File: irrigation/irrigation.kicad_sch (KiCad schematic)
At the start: 37 parts, among them J1 24V Jmp, J10 24V, J11 25%, J12 50%, J13 75%, J14 100%, J15 100%, J16 100%, J17 Pump, J2 Power, J3 Power, J4 Power, J5 Power, J6 Power, J7 Power, J8 0V Jmp, J9 Empty, K1 PLC-RPT-24DC/21, K2 PLC-RPT-24DC/21, M1 Pump, SW1 Well Empty, SW2 100% Full, SW3 25% Full, SW4 50% Full, SW5 75% Full, U1 MPPT-Charger

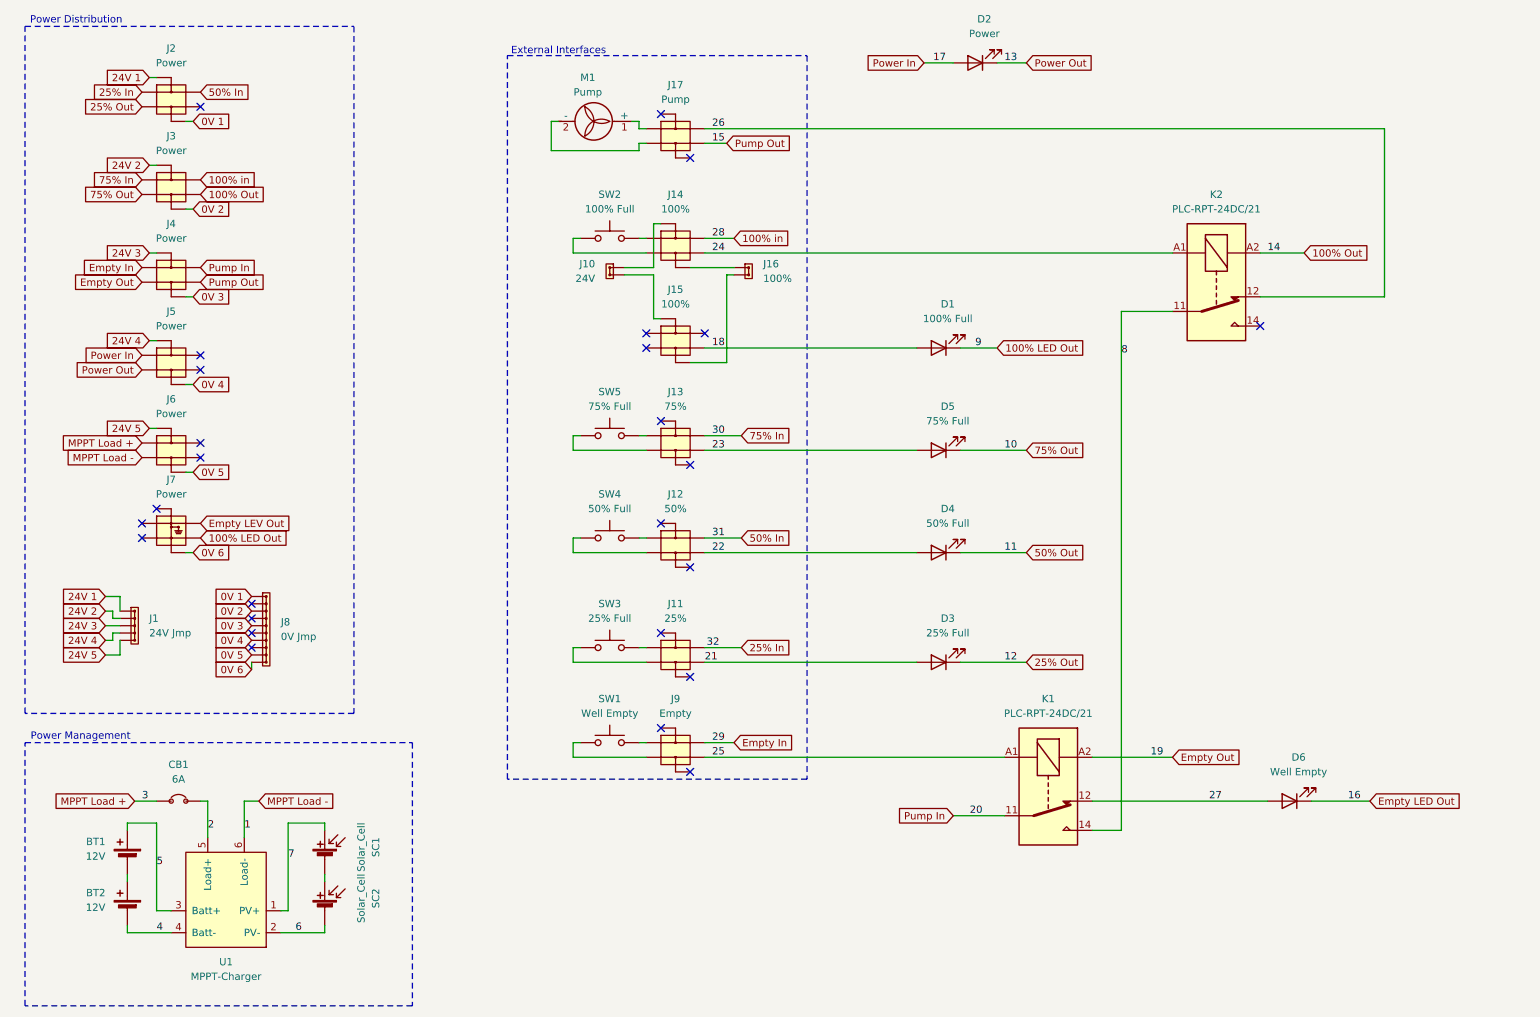
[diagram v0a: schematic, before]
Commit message: Attempting to organize
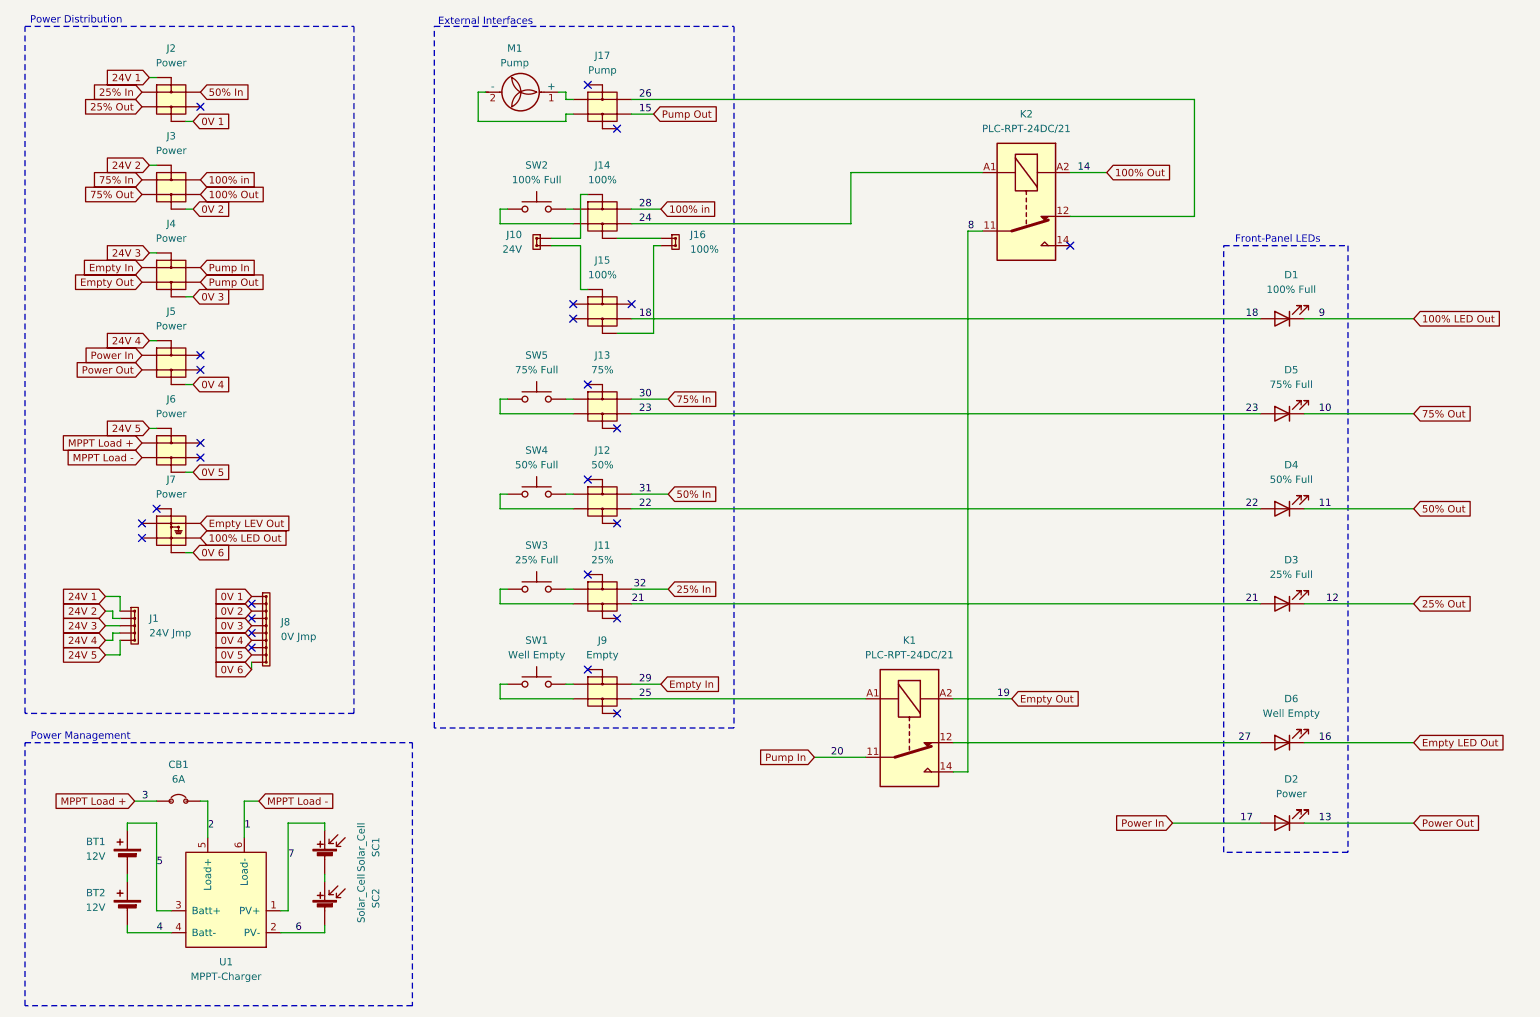
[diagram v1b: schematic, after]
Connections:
- net at J10.: now also J15.; no longer J14.
- net at J16.: now also J15.; no longer J14.
- new net: J10., J14.
- new net: J14., J16.
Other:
- note added: "Front-Panel LEDs"
- moved on the sheet: D1, D2, D3, D4, D5, D6, J10, J11, J12, J13, J14, J15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

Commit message: Organization
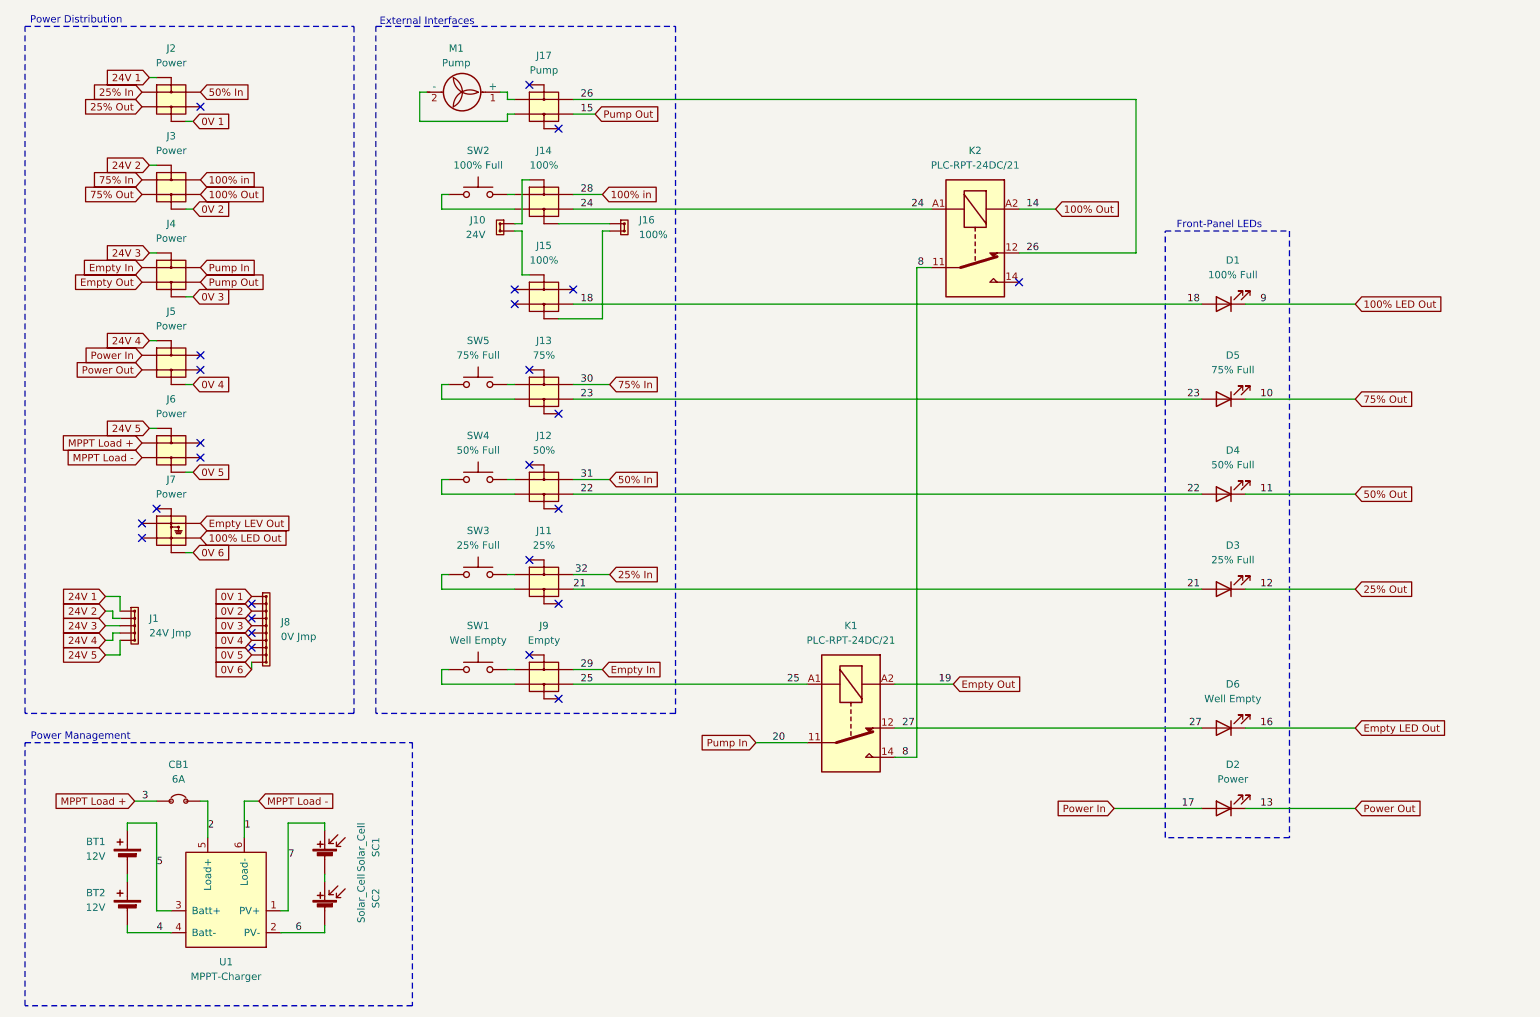
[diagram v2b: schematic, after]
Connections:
- net at J10.: now also J15.; no longer J14.
- net at J16.: now also J15.; no longer J14.
- new net: J10., J14.
- new net: J14., J16.
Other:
- moved on the sheet: D1, D2, D3, D4, D5, D6, J10, J11, J12, J13, J14, J15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
